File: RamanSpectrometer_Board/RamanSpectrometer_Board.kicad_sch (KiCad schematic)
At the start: 32 parts, among them J1 RJ45_LED_Shielded, Q1 BSS138, Q2 BSS138, Q3 BSS138, Q5 BSS138, U1 Teensy4.1_DEV-16771, U2 OKI 12V-5V, U3 OKI 5V-3V

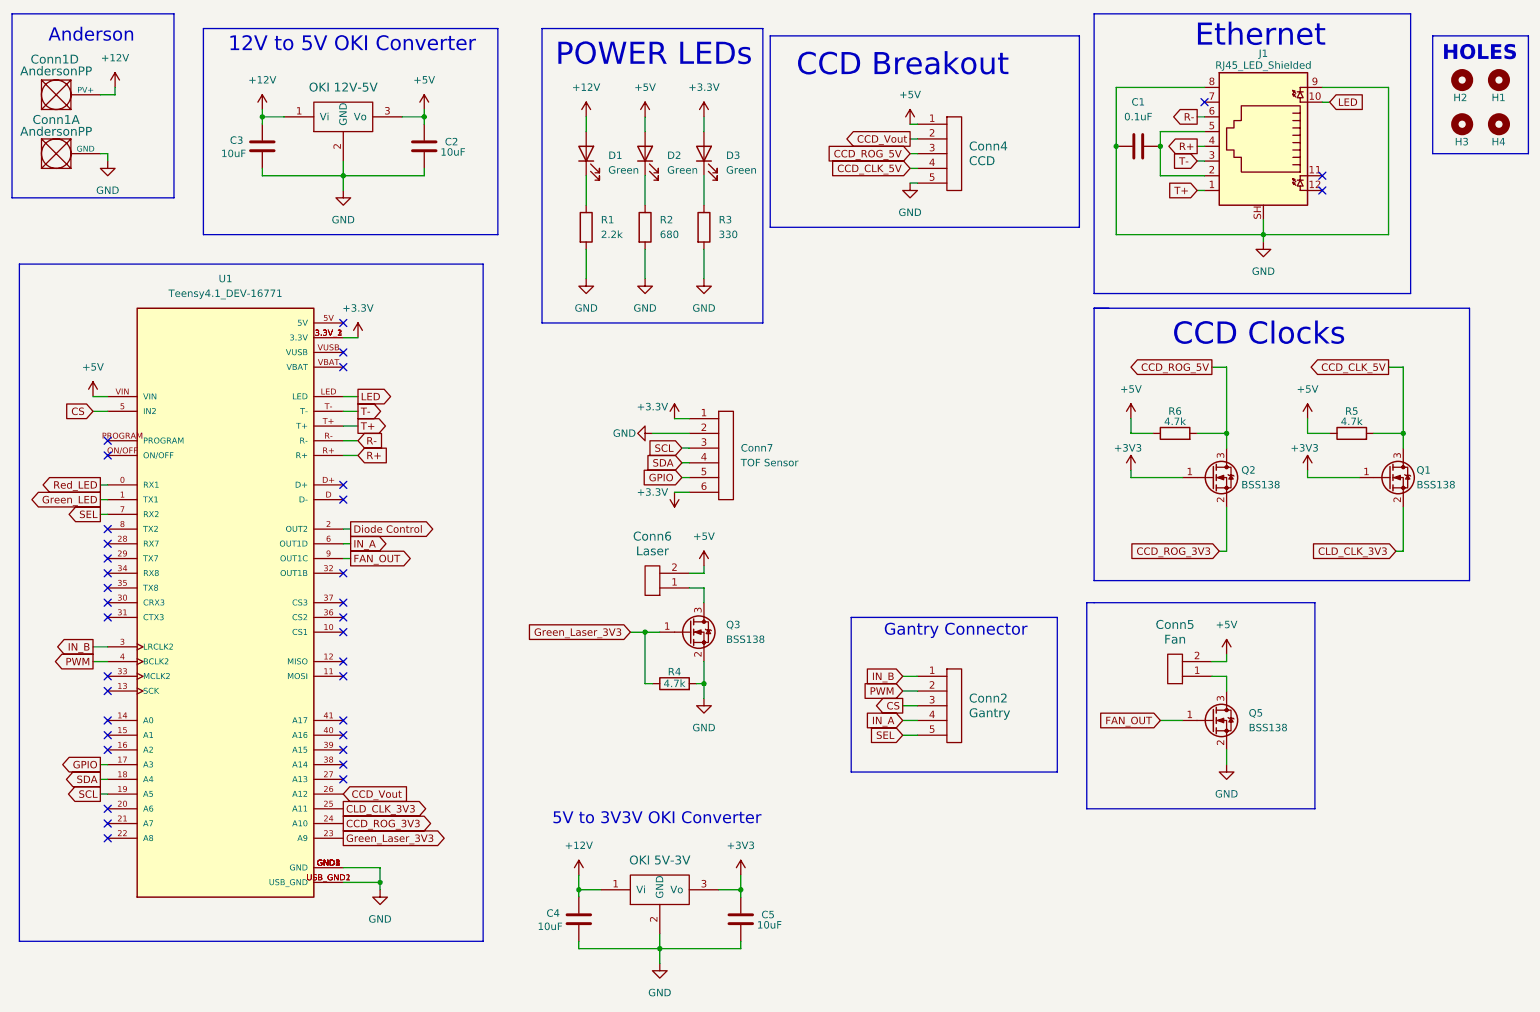
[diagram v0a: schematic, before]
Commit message: Schematic Changes
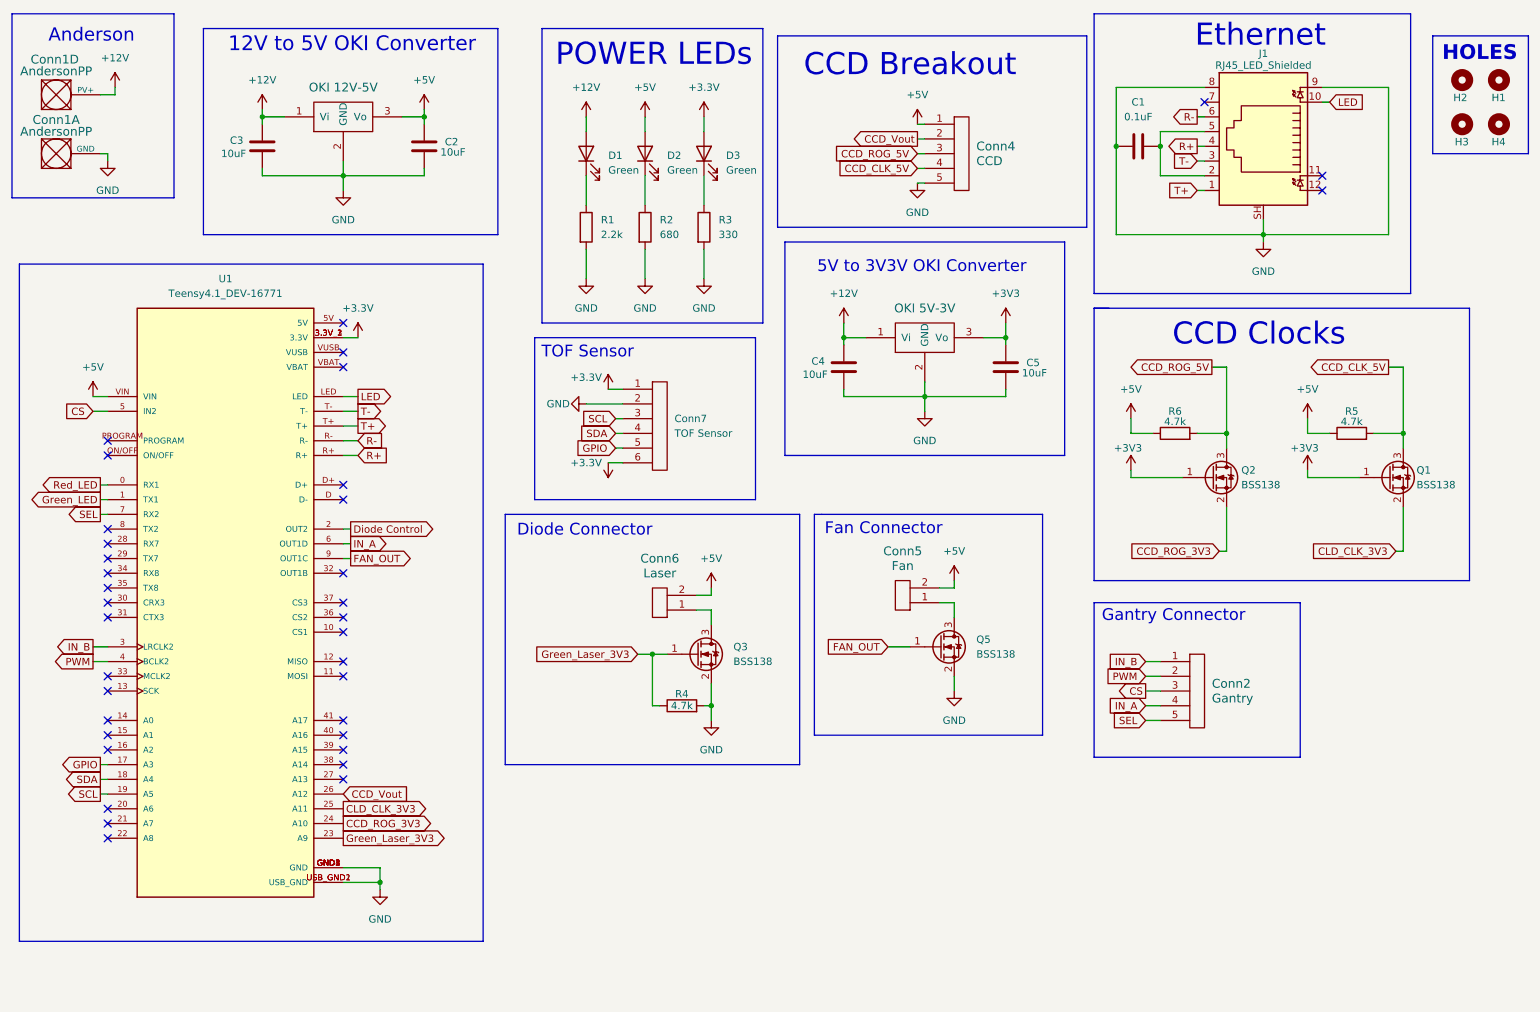
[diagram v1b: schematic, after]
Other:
- note added: "Diode Connector"
- note added: "Fan Connector"
- note added: "TOF Sensor"
- moved on the sheet: C4, C5, Conn2, Conn4, Conn5, Conn6, Conn7, Q3, Q5, R4
